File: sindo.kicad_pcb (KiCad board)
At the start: 2 copper layers, 153 parts, among them J1 Conn_02x06_Top_Bottom, J2 Conn_02x06_Top_Bottom, U1 ESP32DEVKITV1

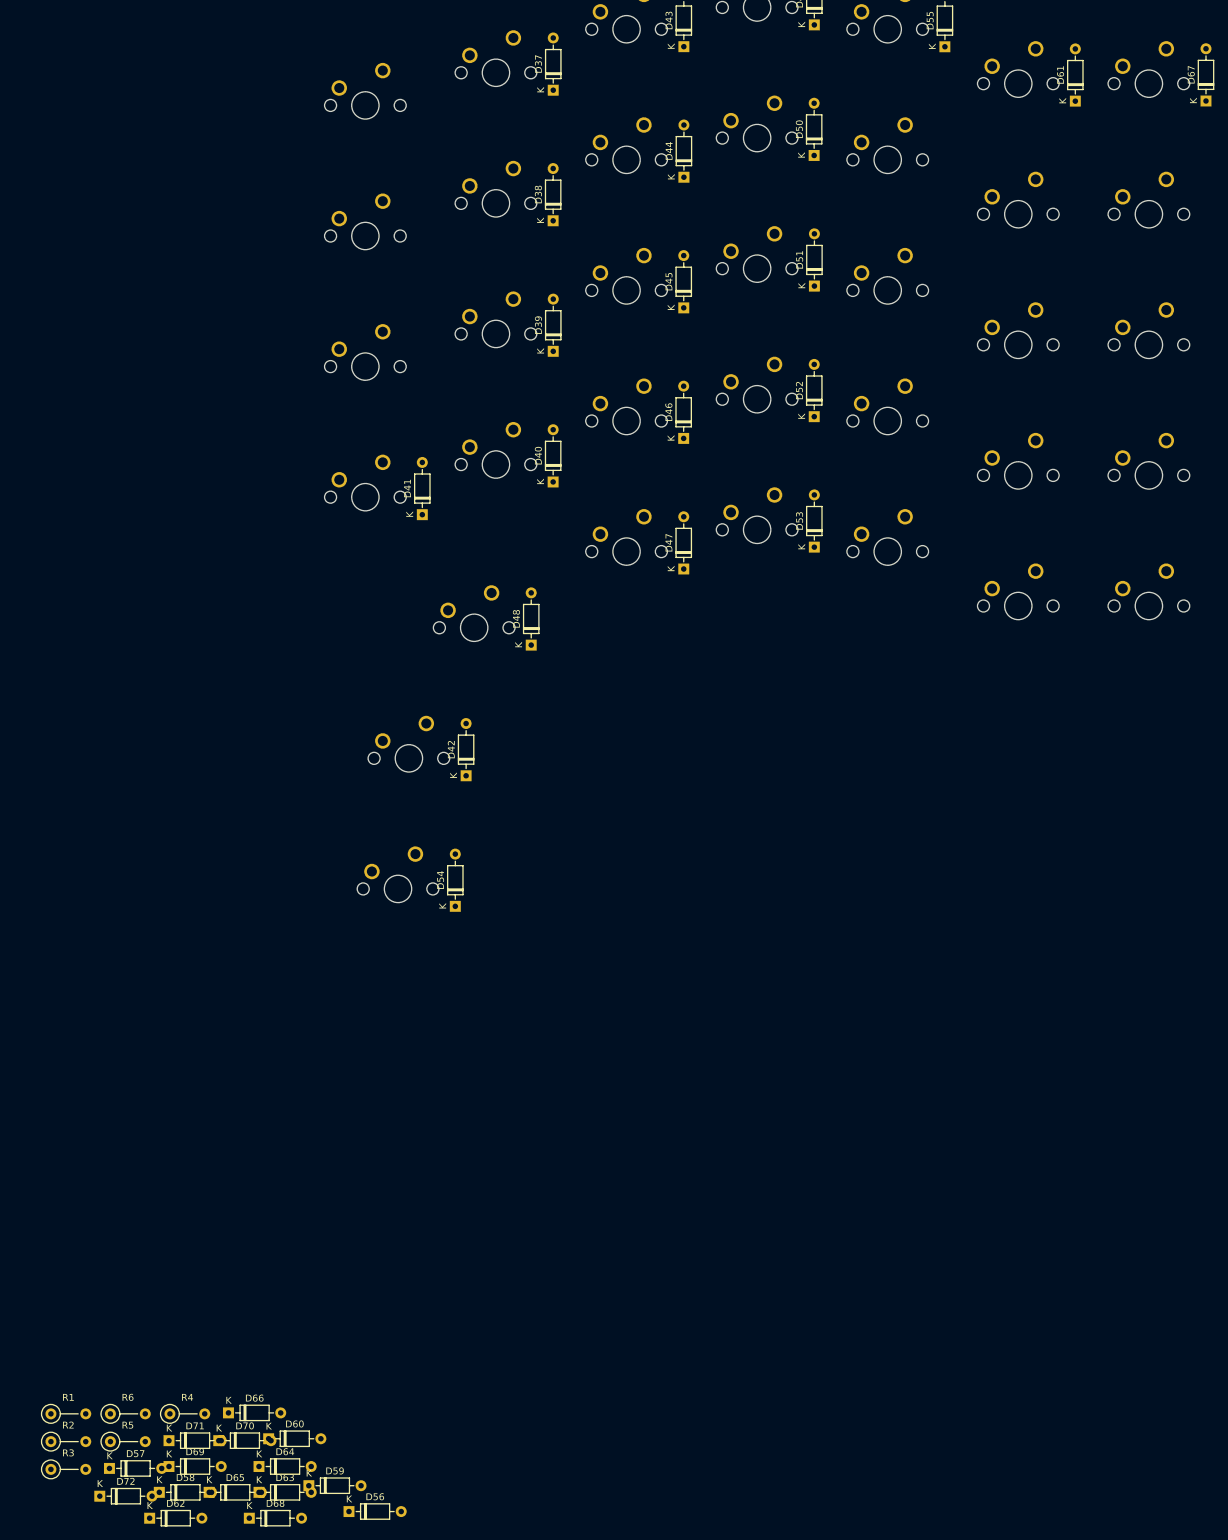
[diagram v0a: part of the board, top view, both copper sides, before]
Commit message: Done with the basic layout
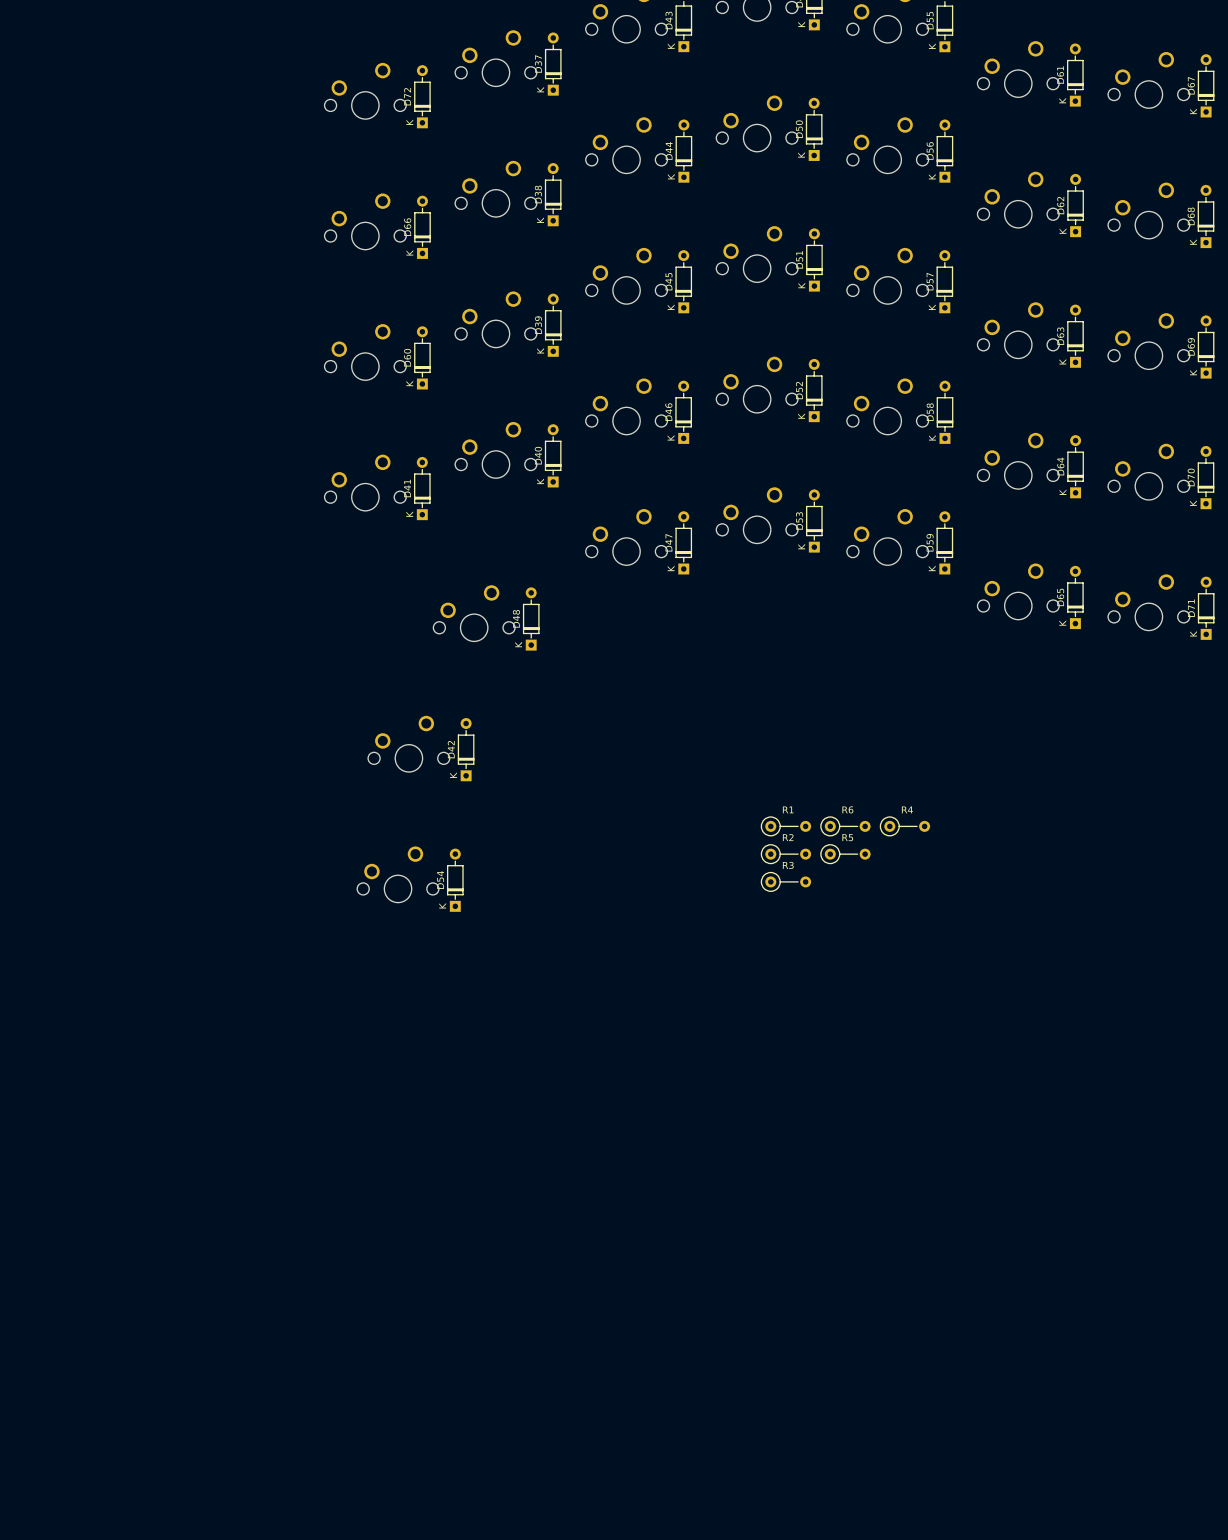
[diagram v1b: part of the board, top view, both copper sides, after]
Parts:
- moved D68 232.6 mm to (141.7, -38.7), turned to 90 degrees
- moved D62 231.2 mm to (122.7, -40.3), turned to 90 degrees
- moved D69 219.8 mm to (141.7, -19.7), turned to 90 degrees
- moved D56 213.2 mm to (103.6, -48.3), turned to 90 degrees
- moved D57 208.6 mm to (103.6, -29.2), turned to 90 degrees
- moved D72 205.8 mm to (27.4, -56.2), turned to 90 degrees
- moved D63 203.4 mm to (122.6, -21.3), turned to 90 degrees
- moved D70 198.6 mm to (141.7, -0.64), turned to 90 degrees
- moved D58 191.8 mm to (103.6, -10.2), turned to 90 degrees
- moved D71 191.6 mm to (141.7, 18.4), turned to 90 degrees
- moved D64 185.4 mm to (122.7, -2.22), turned to 90 degrees
- moved D65 179.0 mm to (122.6, 16.9), turned to 90 degrees
- moved D66 171.5 mm to (27.4, -37.1), turned to 90 degrees
- moved D59 162.8 mm to (103.6, 8.89), turned to 90 degrees
- moved D60 155.5 mm to (27.4, -18.1), turned to 90 degrees
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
